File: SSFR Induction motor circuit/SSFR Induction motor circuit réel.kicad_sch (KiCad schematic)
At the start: 24 parts, among them U1 LM741, U2 LM741, U3 LM741, U4 ESP32-WROOM-32, U5 LM741

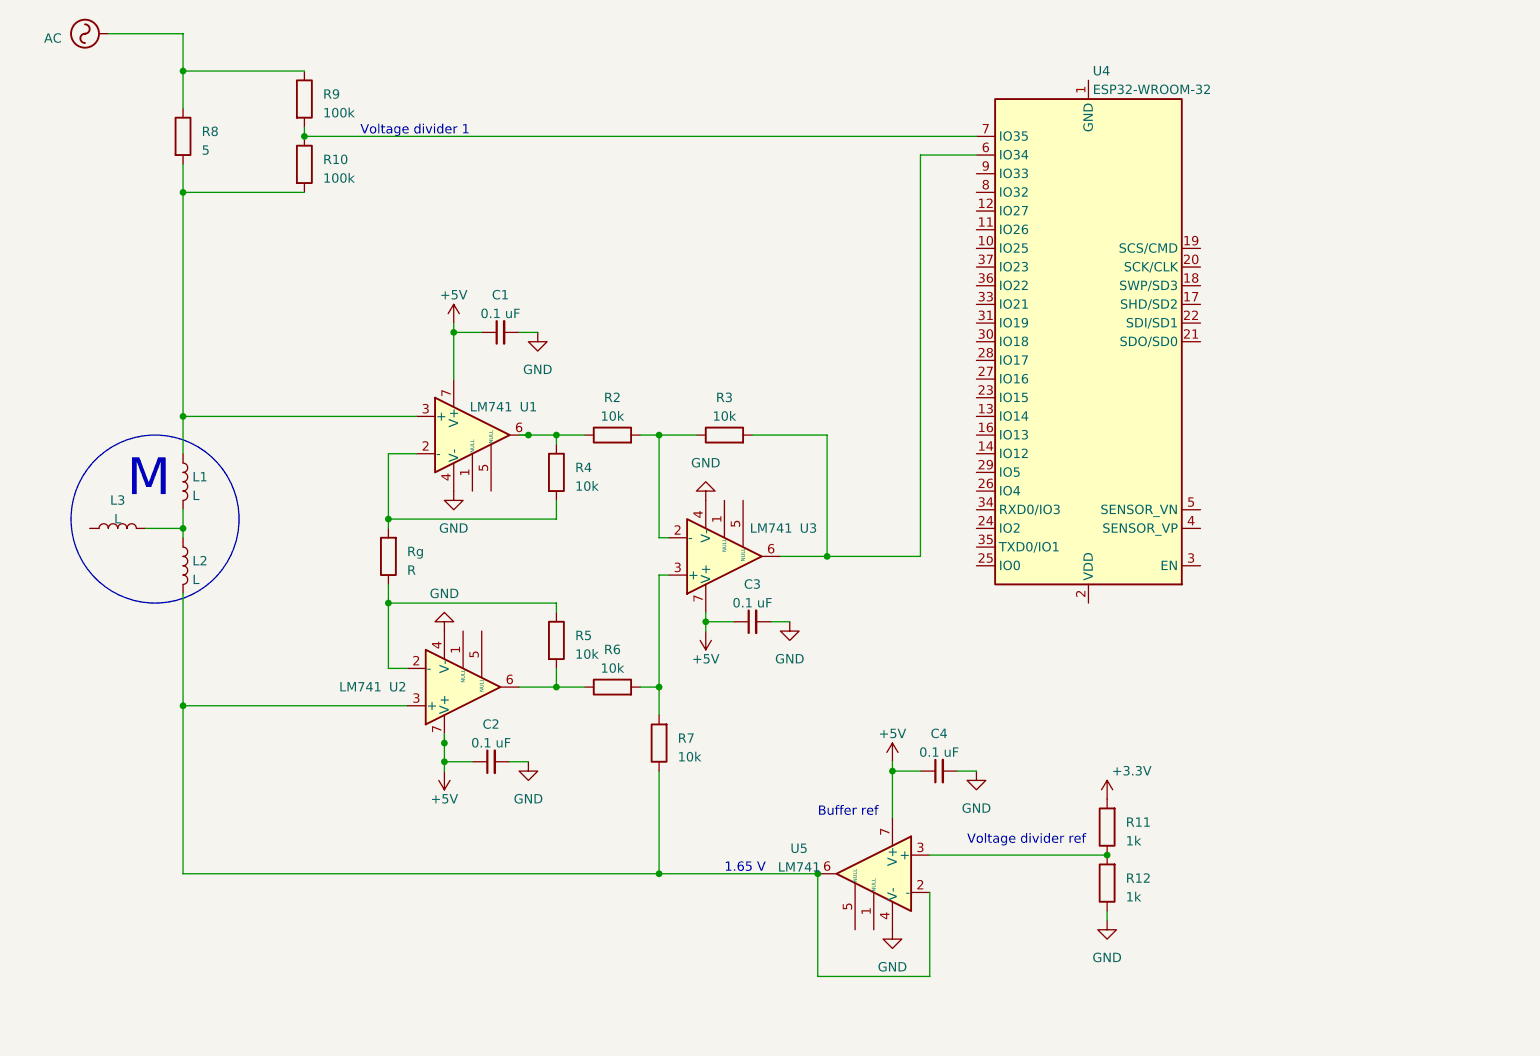
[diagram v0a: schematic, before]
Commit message: update du circuit et du code
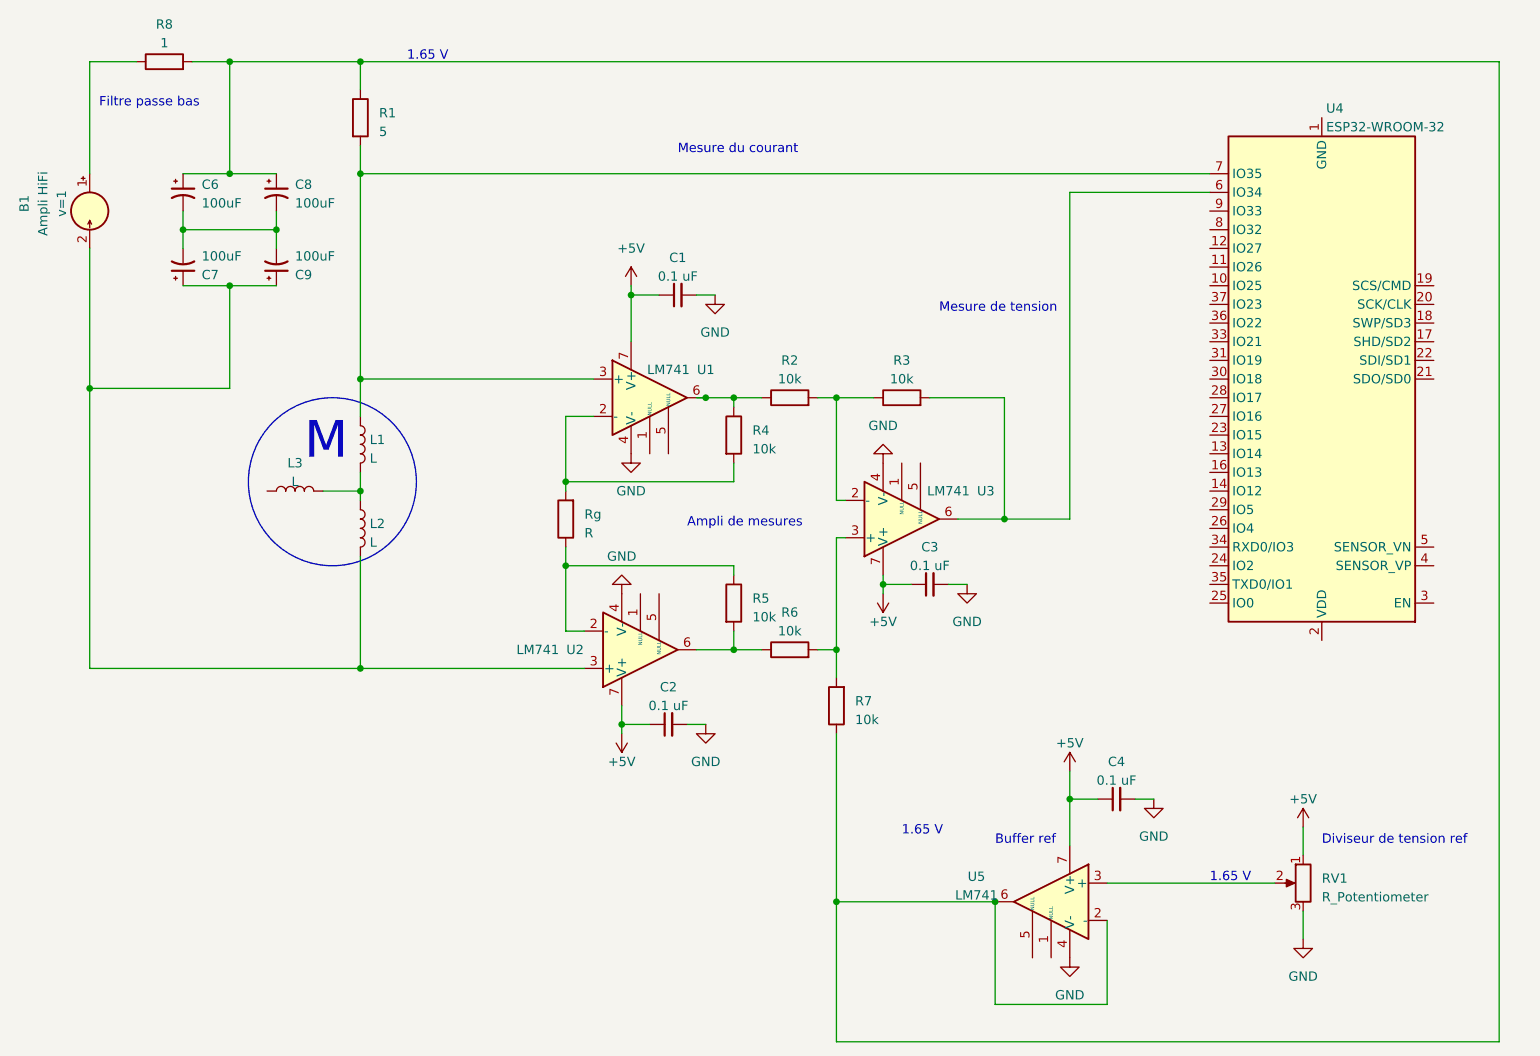
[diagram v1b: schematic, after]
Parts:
- removed R10, R9: 100k, symbol Device:R
- removed R11, R12: 1k, symbol Device:R
- added B1: Ampli HiFi, symbol Simulation_SPICE:BSOURCE
- added C6, C7, C8, C9: 100uF, symbol Device:C_Polarized_Small_US
- added R1: 5, symbol Device:R
- added RV1: R_Potentiometer, symbol Device:R_Potentiometer
- R8: value 5 -> 1
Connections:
- net +5V: now also RV1.1
- net GND: now also RV1.3
- net at R7.1, U5.2 (-), U5.6: now also R8.2, C6.1, C8.1, R1.1; no longer L2.2, U2.3 (+)
- net at U4.7 (IO35): now also L1.1, U1.3 (+), R1.2
- net at U5.3 (+): now also RV1.2
- net AC: no longer names the net of R8.1
- net AC: now also B1.1 (N+)
- new net: B1.2 (N-), C7.1, C9.1, L2.2, U2.3 (+)
- new net: C6.2, C7.2, C8.2, C9.2
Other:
- note added: "Ampli de mesures"
- note added: "Diviseur de tension ref"
- note added: "Filtre passe bas"
- note added: "Mesure de tension"
- note added: "Mesure du courant"
- note removed: "Voltage divider 1"
- note removed: "Voltage divider ref"
- moved on the sheet: C1, C2, C3, C4, L1, L2, L3, R2, R3, R4, R5, R6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
